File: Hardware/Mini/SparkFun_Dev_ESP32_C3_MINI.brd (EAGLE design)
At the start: 17.8 x 33 mm, 44 parts, among them J1 USB Female Type C Connector, J5 Vertical Qwiic Connector, U2 RT9080-33GJ5

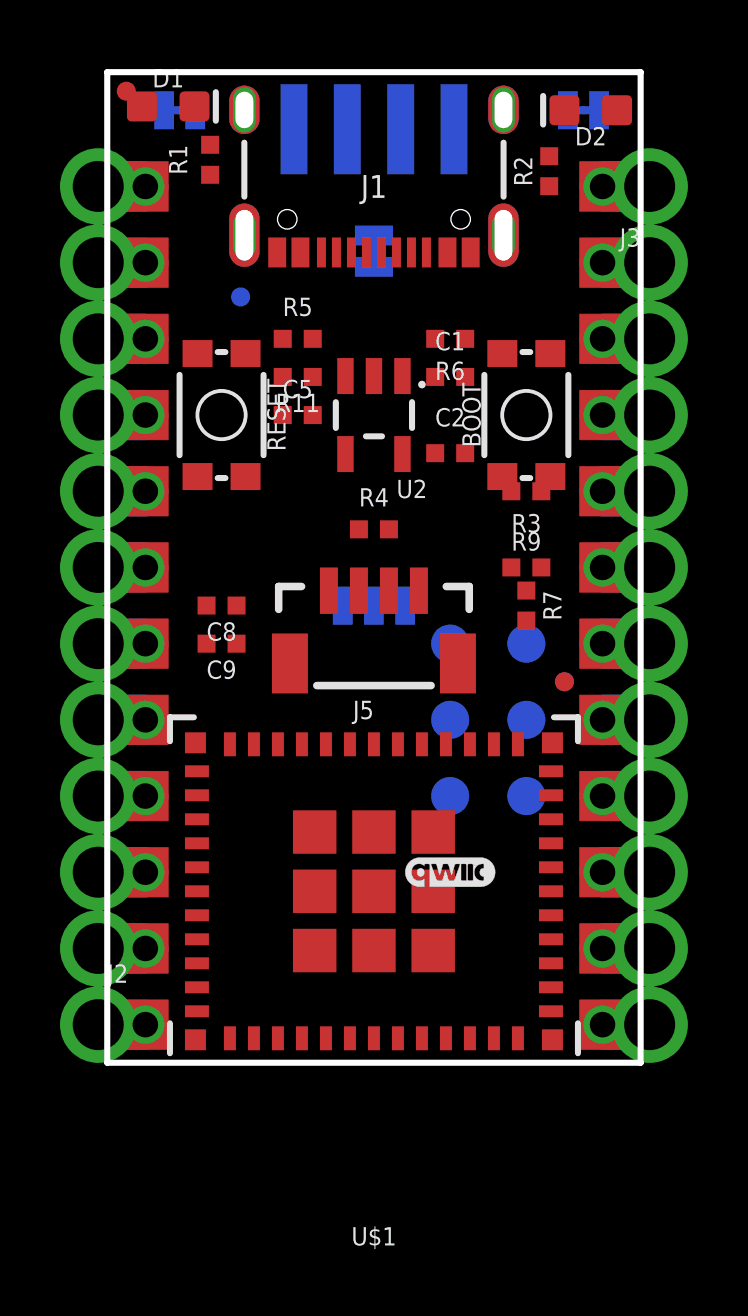
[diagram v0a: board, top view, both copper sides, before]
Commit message: Moves some parts away as lost in thought
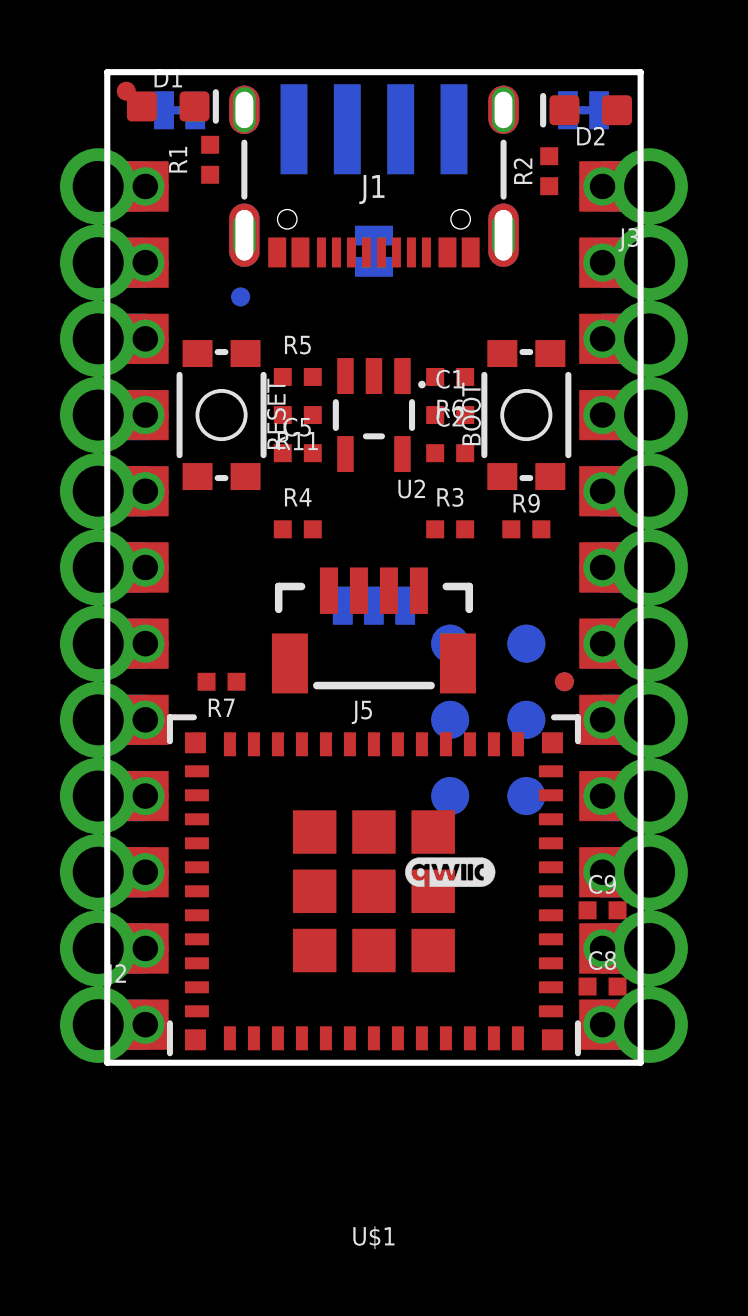
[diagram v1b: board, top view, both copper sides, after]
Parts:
- moved C8 18.0 mm to (17.8, 2.54), turned to 0 degrees
- moved C9 15.5 mm to (17.8, 5.08), turned to 0 degrees
- moved R7 10.5 mm to (5.08, 12.7), turned to 180 degrees
- moved R3 2.84 mm to (12.7, 17.8), turned to 0 degrees
- moved R4 2.54 mm to (7.62, 17.8)
- moved C1 1.27 mm to (12.7, 21.6)
- moved C5 1.27 mm to (7.62, 20.3)
- moved R11 1.27 mm to (7.62, 21.6)
- moved R5 1.27 mm to (7.62, 22.9)
- moved R6 1.27 mm to (12.7, 22.9)
- moved R9 1.27 mm to (15.2, 17.8)
